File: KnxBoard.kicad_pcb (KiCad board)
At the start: 4 copper layers, 35.8 x 33.5 mm, 41 parts, among them IC1 STM32G491KEU6, IC2 NCN5130MNTWG, J1 Conn_01x02, J2 Conn_02x03_Counter_Clockwise, J3 Conn_01x10, J4 Conn_01x10, SW1 SW_Push, Y1 16MHz

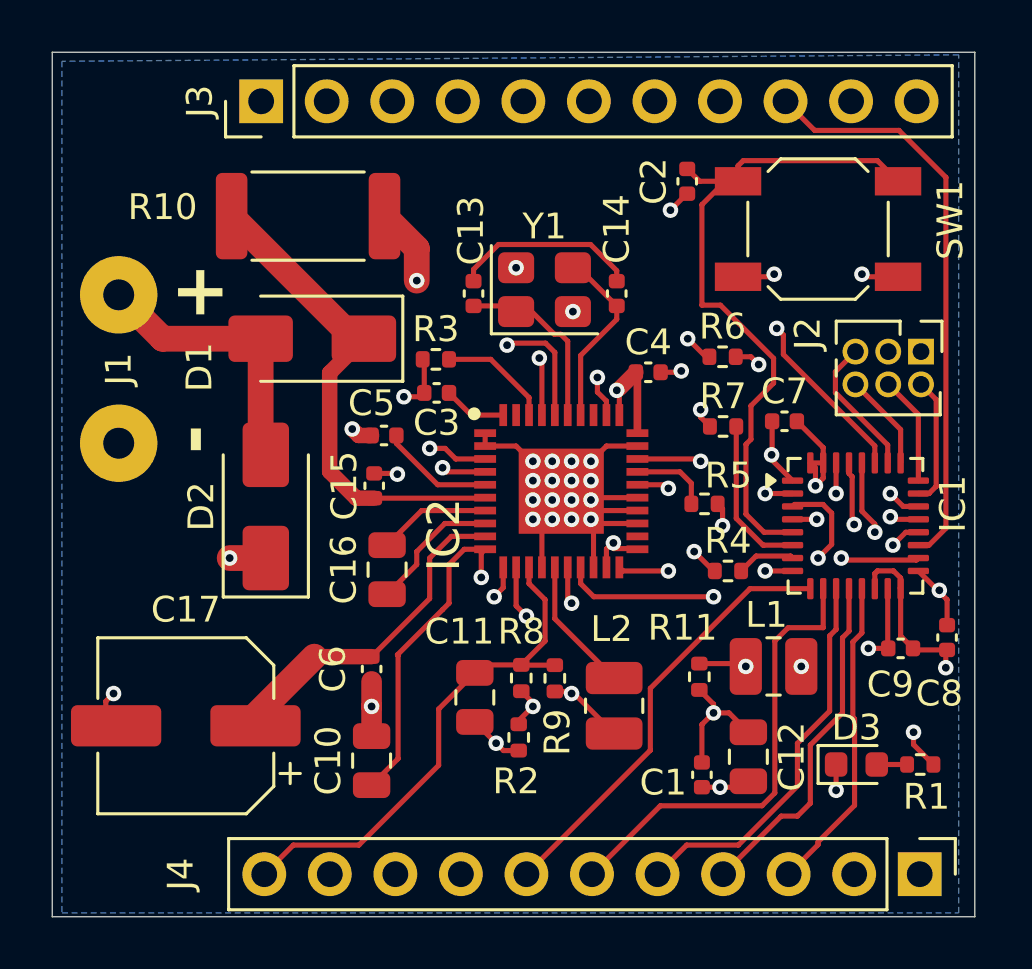
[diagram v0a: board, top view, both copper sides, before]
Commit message: Update size
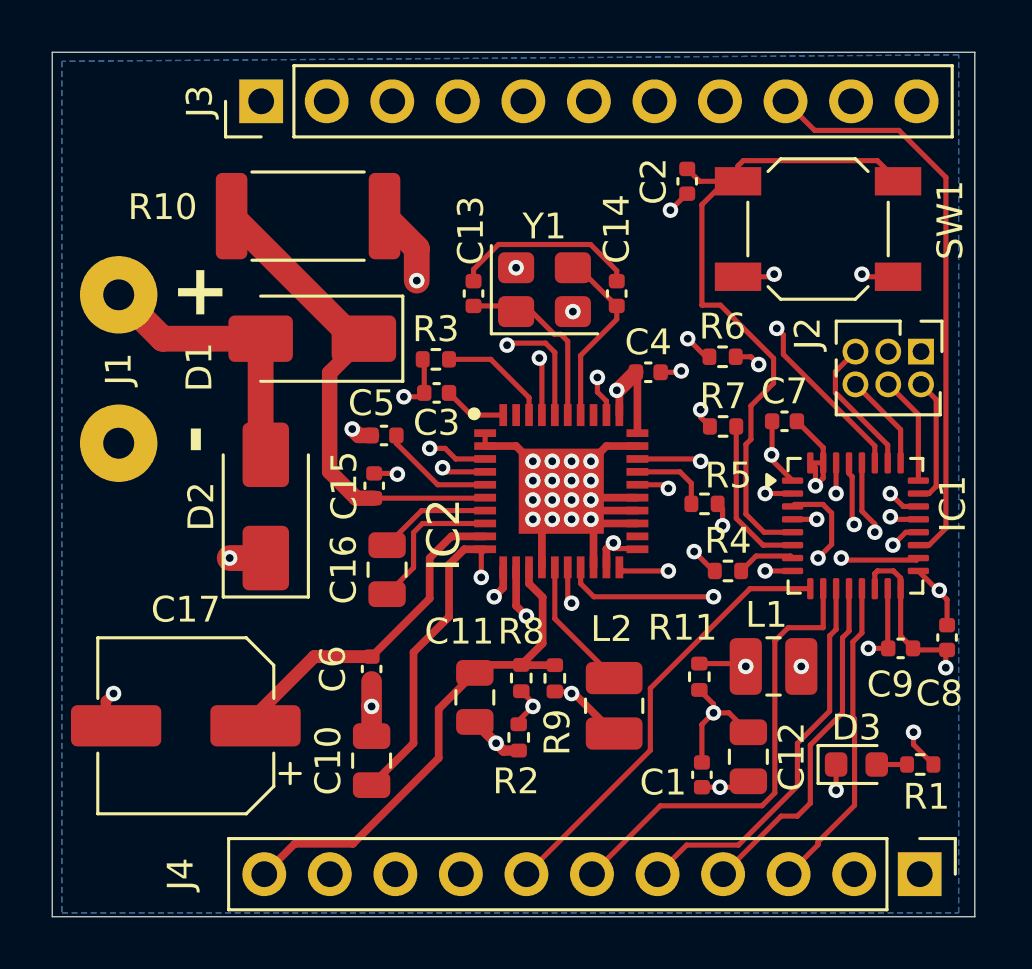
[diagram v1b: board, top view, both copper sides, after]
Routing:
- net Net-(IC2-CEQ2): track 5.23 -> 5.73 mm
